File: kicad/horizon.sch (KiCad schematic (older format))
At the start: 108 parts, among them J1 OLED, SW1 SW_Push, SW10 SW_Push, SW11 SW_Push, SW12 SW_Push, SW13 SW_Push, SW14 SW_Push, SW15 SW_Push, SW16 SW_Push, SW17 SW_Push, SW18 SW_Push, SW19 SW_Push, SW2 SW_Push, SW20 SW_Push, SW21 SW_Push, SW22 SW_Push, SW23 SW_Push, SW24 SW_Push, SW25 SW_Push, SW26 SW_Push, SW27 SW_Push, SW28 SW_Push, SW29 SW_Push, SW3 SW_Push, SW30 SW_Push, SW31 SW_Push, SW32 SW_Push, SW33 SW_Push, SW34 SW_Push, SW35 SW_Push, SW36 SW_Push, SW37 SW_Push, SW38 SW_Push, SW39 SW_Push, SW4 SW_Push, SW40 SW_Push, SW41 SW_Push, SW42 SW_Push, SW43 SW_Push, SW44 SW_Push, SW45 SW_Push, SW46 SW_Push, SW47 SW_Push, SW48 SW_Push, SW49 SW_Push, SW5 SW_Push, SW50 SW_Push, SW6 SW_Push, SW7 SW_Push, SW8 SW_Push, SW9 SW_Push, U1 Pro-Micro

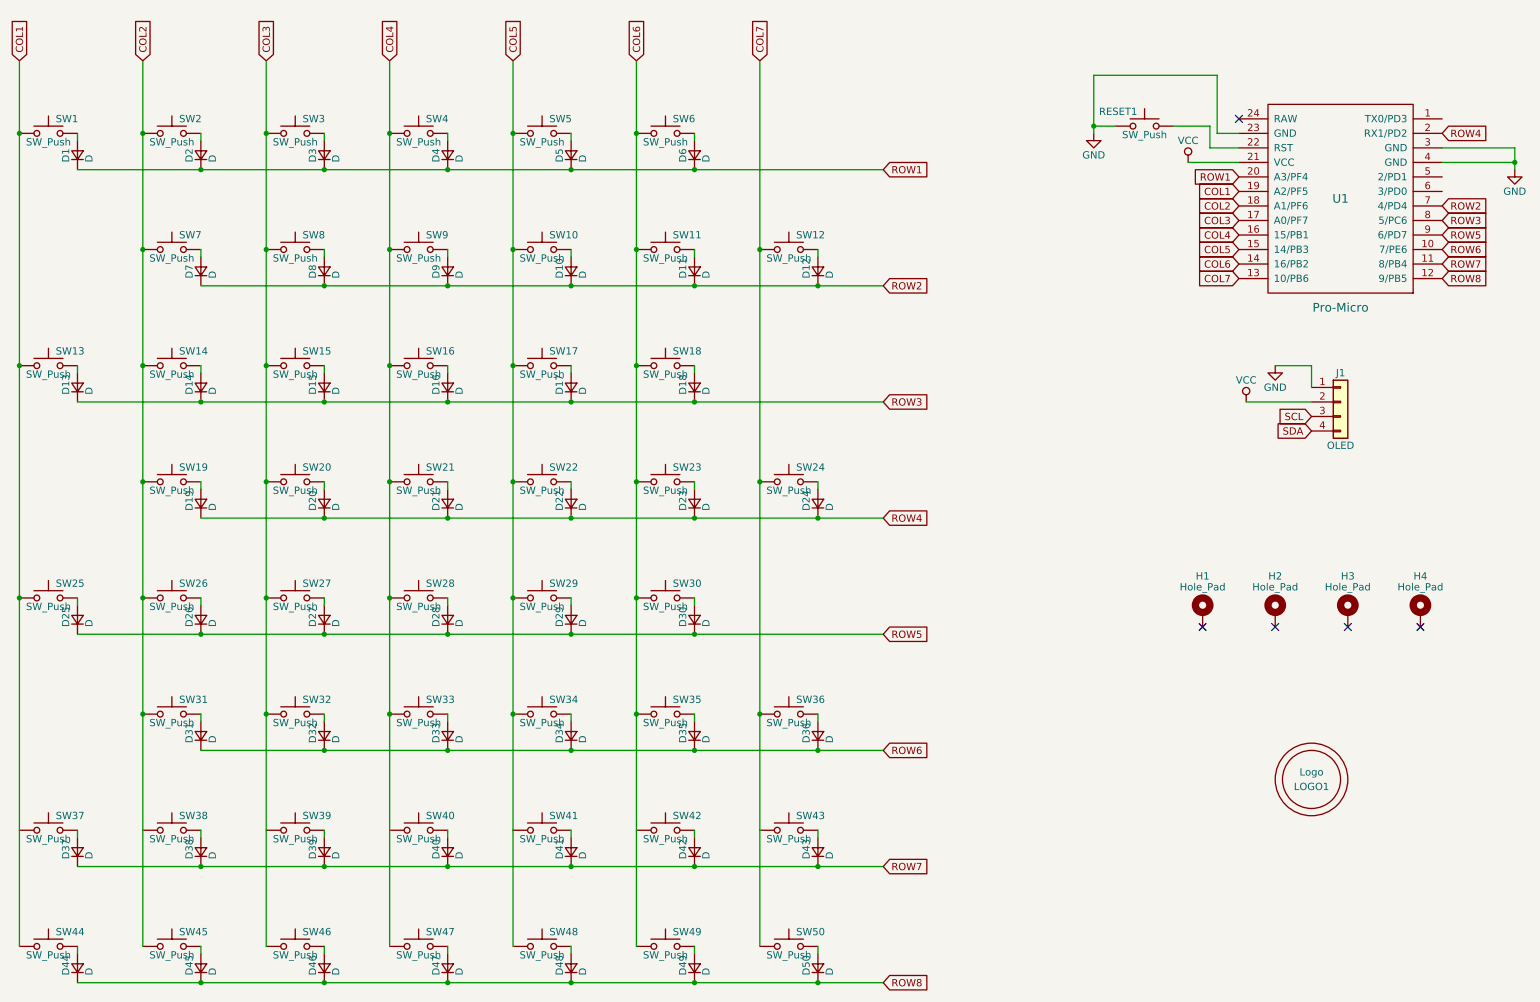
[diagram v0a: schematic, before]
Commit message: Layout MX PCB
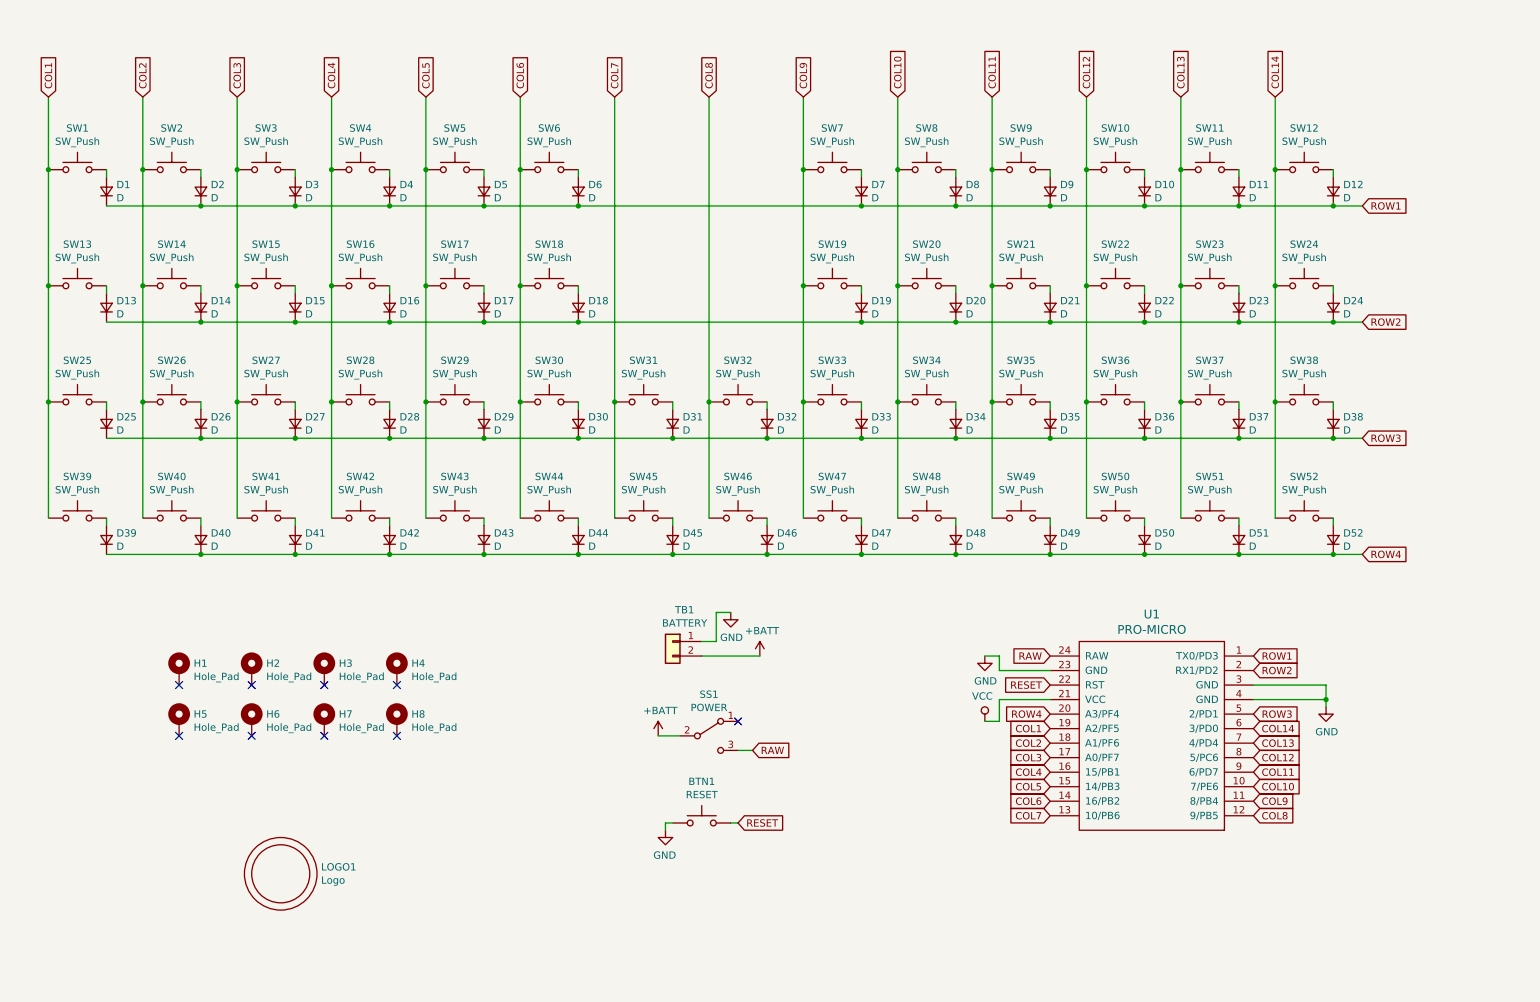
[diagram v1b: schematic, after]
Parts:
- removed J1: OLED, horizon-footprints:Header_1x04_2.54mm, symbol horizon-components:Conn_01x04
- added D51, D52: D, horizon-footprints:D_SOD-123, symbol horizon-components:D
- added H5, H6, H7, H8: Hole_Pad, horizon-footprints:Mount_M2, symbol horizon-components:Hole_Pad
- added SS1: POWER, horizon-footprints:SS12D00, symbol horizon-components:SW_SPDT
- added SW51, SW52: SW_Push, horizon-footprints:SW_MX, symbol horizon-components:SW_Push
- added TB1: BATTERY, horizon-footprints:KF350-2P, symbol horizon-components:Conn_01x02
- BTN1: renamed from RESET1; value SW_Push -> RESET
- LOGO1: footprint horizon-footprints:Logo_Horizon -> horizon-footprints:Logo_Horizon_Small
- U1: value Pro-Micro -> PRO-MICRO
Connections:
- net COL1: now also SW39.1; no longer SW37.1, SW44.1
- net COL2: now also SW40.1; no longer SW19.1, SW31.1, SW38.1, SW45.1, SW7.1
- net COL3: now also SW41.1; no longer SW20.1, SW32.1, SW39.1, SW46.1, SW8.1
- net COL4: now also SW42.1; no longer SW21.1, SW33.1, SW40.1, SW47.1, SW9.1
- net COL5: now also SW43.1; no longer SW10.1, SW22.1, SW34.1, SW41.1, SW48.1
- net COL6: now also SW44.1; no longer SW11.1, SW23.1, SW35.1, SW42.1, SW49.1
- net COL7: now also SW31.1, SW45.1; no longer SW12.1, SW24.1, SW36.1, SW43.1, SW50.1
- net GND: now also TB1.1 (Pin_1)
- net ROW1: now also D10.1 (K), D11.1 (K), D12.1 (K), D7.1 (K), D8.1 (K), D9.1 (K), U1.1 (TX0/PD3); no longer U1.20 (A3/PF4)
- net ROW2: now also D13.1 (K), D14.1 (K), D15.1 (K), D16.1 (K), D17.1 (K), D18.1 (K), D19.1 (K), D20.1 (K), D21.1 (K), D22.1 (K), D23.1 (K), D24.1 (K), U1.2 (RX1/PD2); no longer D10.1 (K), D11.1 (K), D12.1 (K), D7.1 (K), D8.1 (K), D9.1 (K), U1.7 (4/PD4)
- net ROW3: now also D25.1 (K), D26.1 (K), D27.1 (K), D28.1 (K), D29.1 (K), D30.1 (K), D31.1 (K), D32.1 (K), D33.1 (K), D34.1 (K), D35.1 (K), D36.1 (K), D37.1 (K), D38.1 (K), U1.5 (2/PD1); no longer D13.1 (K), D14.1 (K), D15.1 (K), D16.1 (K), D17.1 (K), D18.1 (K), U1.8 (5/PC6)
- net ROW4: now also D39.1 (K), D40.1 (K), D41.1 (K), D42.1 (K), D43.1 (K), D44.1 (K), D45.1 (K), D46.1 (K), D47.1 (K), D48.1 (K), D49.1 (K), D50.1 (K), U1.20 (A3/PF4), D51.1 (K), D52.1 (K); no longer D19.1 (K), D20.1 (K), D21.1 (K), D22.1 (K), D23.1 (K), D24.1 (K), U1.2 (RX1/PD2)
- net RESET: now reaches BTN1.1, U1.22 (RST)
- net RAW: now reaches U1.24 (RAW)
- net RAW: now also SS1.3 (C)
- net COL14: now reaches U1.6 (3/PD0)
- net COL14: now also SW12.1, SW24.1, SW38.1, SW52.1
- removed net ROW5: D25.1 (K), D26.1 (K), D27.1 (K), D28.1 (K), D29.1 (K), D30.1 (K), U1.9 (6/PD7)
- removed net ROW6: D31.1 (K), D32.1 (K), D33.1 (K), D34.1 (K), D35.1 (K), D36.1 (K), U1.10 (7/PE6)
- removed net ROW7: D37.1 (K), D38.1 (K), D39.1 (K), D40.1 (K), D41.1 (K), D42.1 (K), D43.1 (K), U1.11 (8/PB4)
- removed net ROW8: D44.1 (K), D45.1 (K), D46.1 (K), D47.1 (K), D48.1 (K), D49.1 (K), D50.1 (K), U1.12 (9/PB5)
- new net: D51.2 (A), SW51.2
- new net: D52.2 (A), SW52.2
- new net +BATT: SS1.2 (B), TB1.2 (Pin_2)
- new net COL10: SW20.1, SW34.1, SW48.1, SW8.1, U1.10 (7/PE6)
- new net COL11: SW21.1, SW35.1, SW49.1, SW9.1, U1.9 (6/PD7)
- new net COL12: SW10.1, SW22.1, SW36.1, SW50.1, U1.8 (5/PC6)
- new net COL13: SW11.1, SW23.1, SW37.1, SW51.1, U1.7 (4/PD4)
- new net COL8: SW32.1, SW46.1, U1.12 (9/PB5)
- new net COL9: SW19.1, SW33.1, SW47.1, SW7.1, U1.11 (8/PB4)
- no-connect marks 5 -> 9
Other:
- moved on the sheet: BTN1, H1, H2, H3, H4, LOGO1, U1
